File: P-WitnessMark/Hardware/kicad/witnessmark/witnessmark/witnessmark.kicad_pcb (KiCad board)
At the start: 2 copper layers, 40 x 90 mm, 46 parts, among them J2 Conn_01x04, J3 Conn_01x11, J4 Conn_01x05, J5 USB_C_Receptacle_USB2.0_16P, U1 STM32U585RITx, U2 AP2112K-3.3, U3 SLS32AIA010MHUSON10XTMA2, U4 USBLC6-2SC6, Y1 SAW31212F58-32.768K

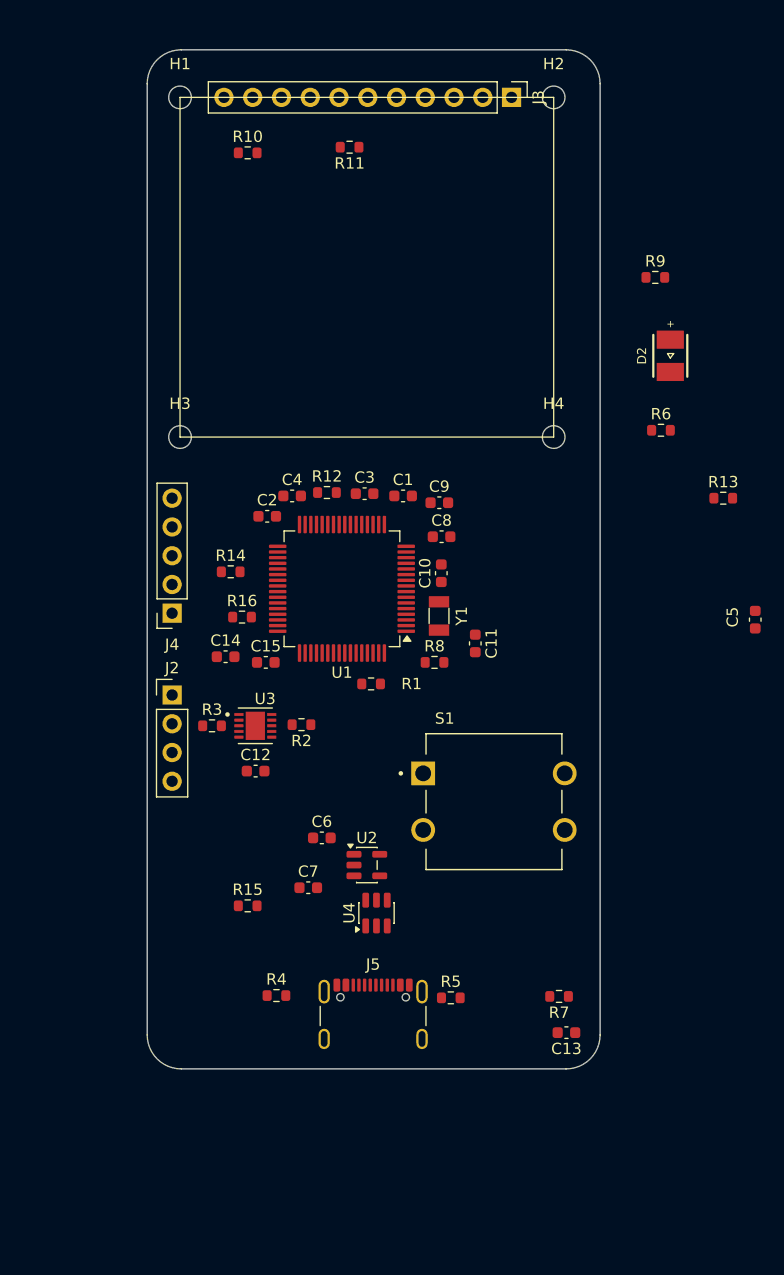
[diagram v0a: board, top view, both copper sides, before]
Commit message: WitnessMark PCB: routed board, 418 segments (promoted from recovery copy)
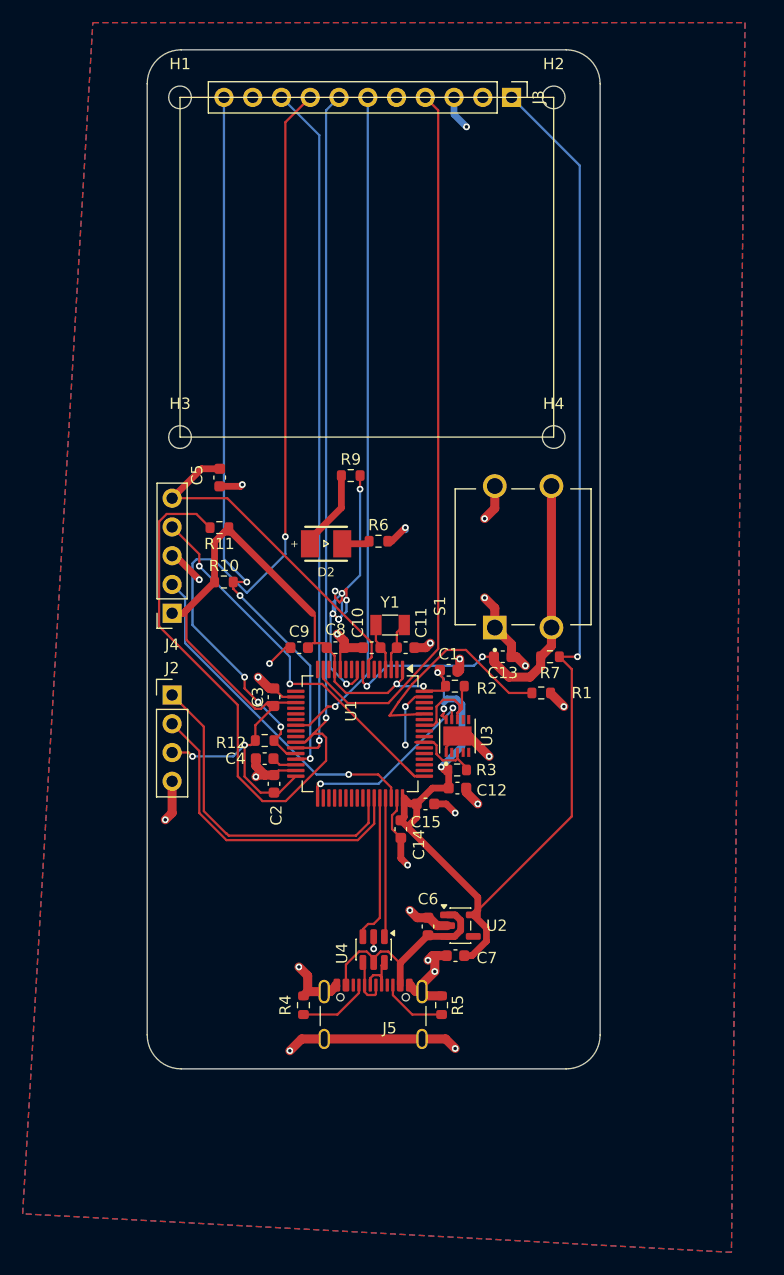
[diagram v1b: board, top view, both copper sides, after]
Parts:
- removed R13, R14, R15, R16, R8: 0Ω, Resistor_SMD:R_0603_1608Metric
- moved C5 48.9 mm to (115.2, 54.2)
- moved R10 38.0 mm to (115.6, 63.4)
- moved R11 35.5 mm to (115.2, 58.6)
- moved D2 34.6 mm to (124.6, 60.0), turned to 180 degrees
- moved C13 33.7 mm to (140.2, 70.0)
- moved R9 32.1 mm to (126.8, 54.0)
- moved R7 30.0 mm to (144.4, 70.0)
- moved R6 26.8 mm to (129.2, 59.8)
- moved C2 23.6 mm to (120.0, 81.2), turned to 90 degrees
- moved C4 23.3 mm to (119.2, 79.0)
- moved R12 22.6 mm to (119.2, 77.4)
- moved R3 22.0 mm to (136.2, 80.0)
- moved S1 21.8 mm to (142.0, 61.2), turned to 90 degrees
- moved C14 21.7 mm to (131.2, 85.2), turned to -90 degrees
- moved C3 19.7 mm to (120.0, 73.6), turned to 90 degrees
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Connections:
- net /Root/+3V3 renamed /+3V3
- net /Root/BOOT0 renamed /BOOT0
- net /Root/CONFIRM_BTN renamed /CONFIRM_BTN
- net /Root/GND renamed /GND
- net /Root/LCD_BL renamed /LCD_BL
- net /Root/LCD_CS renamed /LCD_CS
- net /Root/LCD_DC renamed /LCD_DC
- net /Root/LCD_MOSI renamed /LCD_MOSI
- net /Root/LCD_RST renamed /LCD_RST
- net /Root/LCD_SCK renamed /LCD_SCK
- net /Root/NRST renamed /NRST
- net /Root/OPTIGA_RST renamed /OPTIGA_RST
- net /Root/OPTIGA_SCL renamed /OPTIGA_SCL
- net /Root/OPTIGA_SDA renamed /OPTIGA_SDA
- net /Root/RCC_OSC32_IN renamed /RCC_OSC32_IN
- net /Root/SCAN_RX renamed /SCAN_RX
- net /Root/SCAN_TX renamed /SCAN_TX
- net /Root/STATUS_LED renamed /STATUS_LED
- net /Root/VBUS renamed /VBUS
- C10 pad 1: /Root/RCC_OSC32_OUT -> /RCC_OSC32_OUT
- J4 pad 2: Net-(J4-Pin_2) -> /DEBUG_JTMS-SWDIO
- J4 pad 4: Net-(J4-Pin_4) -> /DEBUG_JTCK-SWCLK
- J5 pad A6: /Root/USB_DP_CONN -> /USB_DP_CONN
- J5 pad A7: /Root/USB_DM_CONN -> /USB_DM_CONN
- J5 pad B6: /Root/USB_DP_CONN -> /USB_DP_CONN
- J5 pad B7: /Root/USB_DM_CONN -> /USB_DM_CONN
- U1 pad 4: Net-(U1-PC15) -> /RCC_OSC32_OUT
- U1 pad 44: Net-(U1-PA11) -> /USB_DM
- U1 pad 45: Net-(U1-PA12) -> /USB_DP
- U1 pad 46: /Root/DEBUG_JTMS-SWDIO -> /DEBUG_JTMS-SWDIO
- U1 pad 49: /Root/DEBUG_JTCK-SWCLK -> /DEBUG_JTCK-SWCLK
- U4 pad 1: /Root/USB_DM -> /USB_DP
- U4 pad 3: /Root/USB_DP -> /USB_DM
- U4 pad 4: /Root/USB_DP_CONN -> /USB_DM_CONN
- U4 pad 6: /Root/USB_DM_CONN -> /USB_DP_CONN
- Y1 pad 2: /Root/RCC_OSC32_OUT -> /RCC_OSC32_OUT
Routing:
- net /+3V3: track 0.00 -> 199.9 mm, vias 0 -> 8
- net /GND: track 0.00 -> 104.3 mm, vias 0 -> 28
- net /LCD_CS: track 0.00 -> 104.2 mm, vias 0 -> 1
- net /LCD_RST: track 0.00 -> 73.8 mm, vias 0 -> 4
- net /LCD_BL: track 0.00 -> 64.5 mm, vias 0 -> 3
- net /LCD_SCK: track 0.00 -> 63.1 mm
- net /LCD_DC: track 0.00 -> 60.8 mm, vias 0 -> 1
- net /LCD_MOSI: track 0.00 -> 59.2 mm, vias 0 -> 1
- net /CONFIRM_BTN: track 0.00 -> 35.8 mm, vias 0 -> 2
- net /DEBUG_JTCK-SWCLK: track 0.00 -> 34.5 mm, vias 0 -> 2
- net /STATUS_LED: track 0.00 -> 32.8 mm, vias 0 -> 8
- net /NRST: track 0.00 -> 30.7 mm
- net /DEBUG_JTMS-SWDIO: track 0.00 -> 30.1 mm, vias 0 -> 1
- net /SCAN_TX: track 0.00 -> 29.5 mm
- net /SCAN_RX: track 0.00 -> 28.2 mm
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- added copper zone on B.Cu, net /GND
- added copper zone on F.Cu, net /GND
